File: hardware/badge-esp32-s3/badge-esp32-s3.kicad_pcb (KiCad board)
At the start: 2 copper layers, 131.5 x 83.5 mm, 161 parts, among them CN1 B4B-PH-SM4-TB (LF)(SN), CN3 HDR-TH_2P-P2.54-V-F, J1 Connector, USB-TYPE-C-16P, J10 Conn_01x02_Socket, J2 Connector, USB-TYPE-C-16P, J3 Conn_01x02_Socket, J4 Conn_01x02_Socket, J5 Conn_01x02_Socket, J6 Conn_01x04_Socket, J7 Conn_01x02_Socket, J8 Conn_01x04_Socket, J9 Conn_01x02_Socket, P1 PH-2A_C2319, P2 FPC 0.5MM 12P Pull type H2.0m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, Q1 SS8050 200-350, Q2 SS8050 200-350, Q3 HL2301A, Q5 DTC114E, SW3 SK-12F04-G050, SW4 TS665CJ, SW5 TS665CJ, SW6 TS665CJ, SW7 TS665CJ, SW8 TS665CJ, SW9 TS665CJ, U1 ESP32-S3-MINI-1-N8, U18 MMA8452QR1_C11360, U19 FH2.54-09-02PZD, U2 NCP167BMX330TBG, U20 2x14_female, U3 CP2102N-A02-GQFN28R, U4 TP4056, U5 TPS63061DSCR, U6 ZX-SH1.0-4PWT

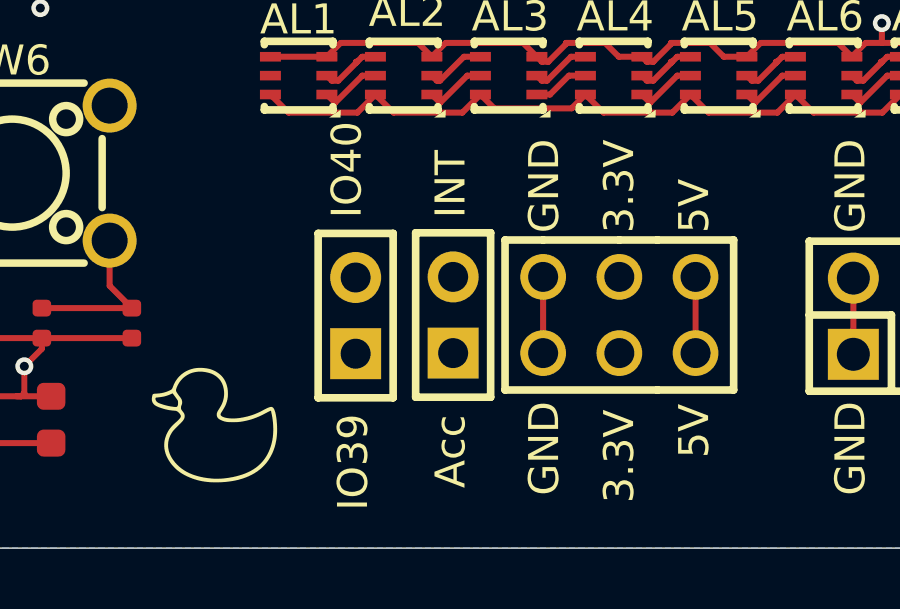
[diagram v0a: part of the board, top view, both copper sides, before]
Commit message: I don't know what changed but I am pushing.
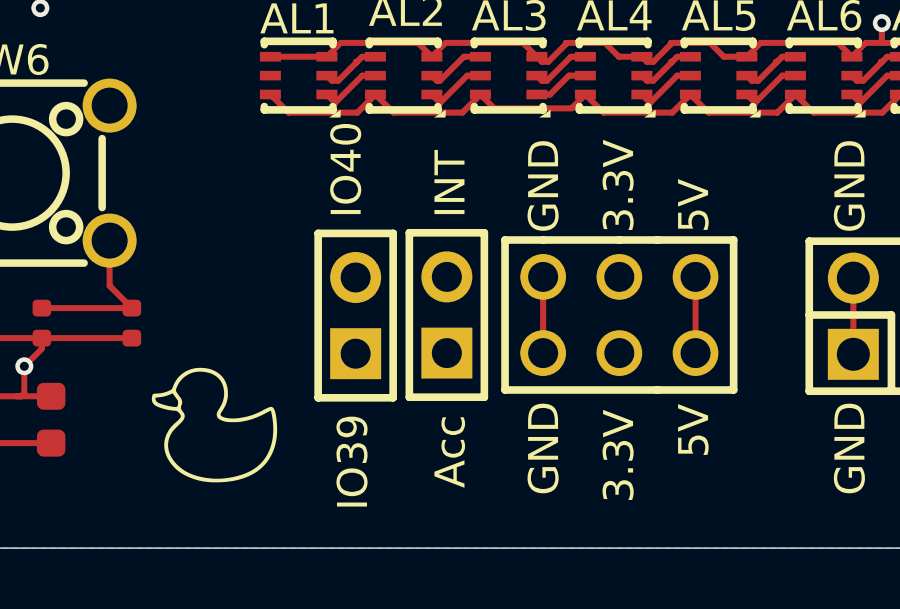
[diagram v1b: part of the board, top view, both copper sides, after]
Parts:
- moved CN2 0.21 mm to (118.2, 138.7)
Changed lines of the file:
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@@
 	(footprint "lcsc-lib:HDR-TH_2P-P2.54-V-F"
 		(layer "F.Cu")
-		(at 118.46 138.73 90)
+		(at 118.25 138.73 90)
 		(property "Reference" "CN2"
 			(at -4.77 -1.5 90)
